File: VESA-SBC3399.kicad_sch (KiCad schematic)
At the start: 0 parts

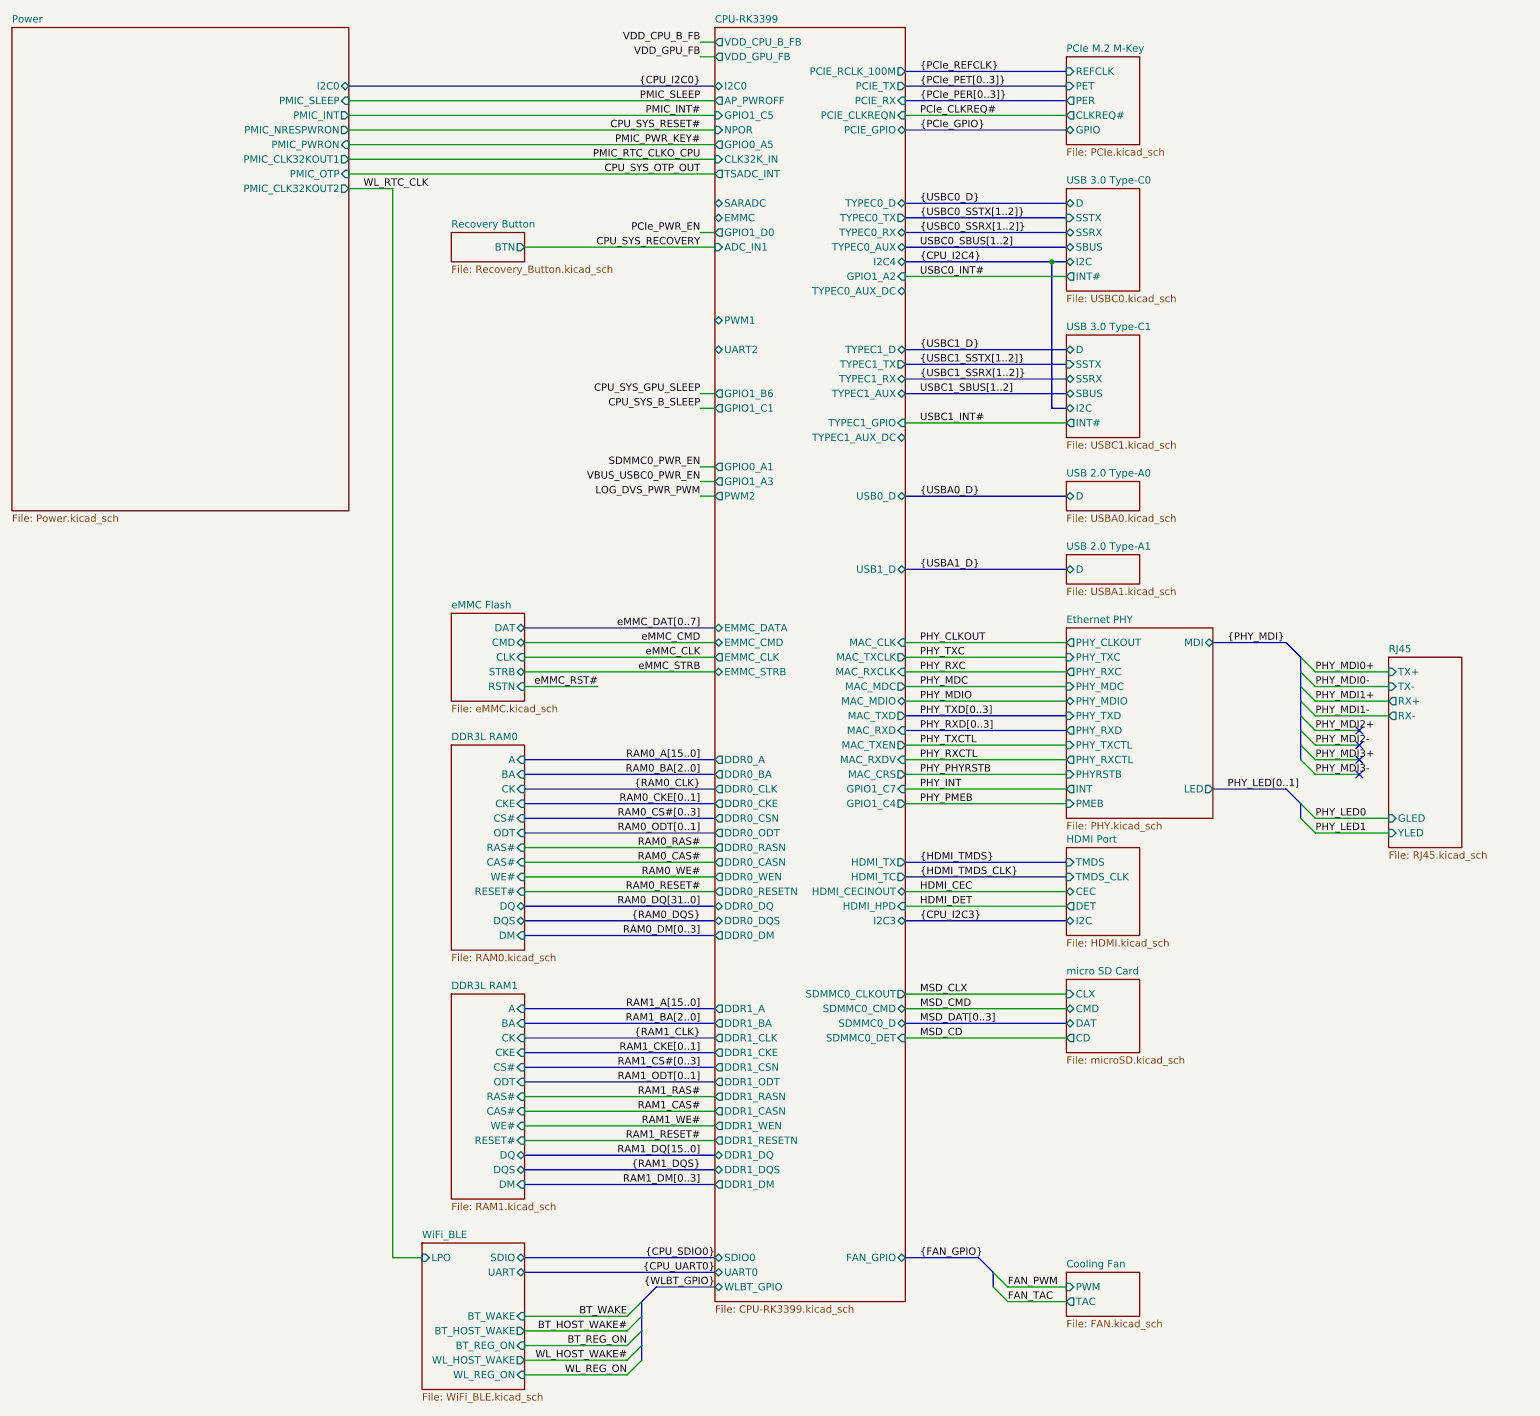
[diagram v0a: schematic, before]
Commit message: update design power
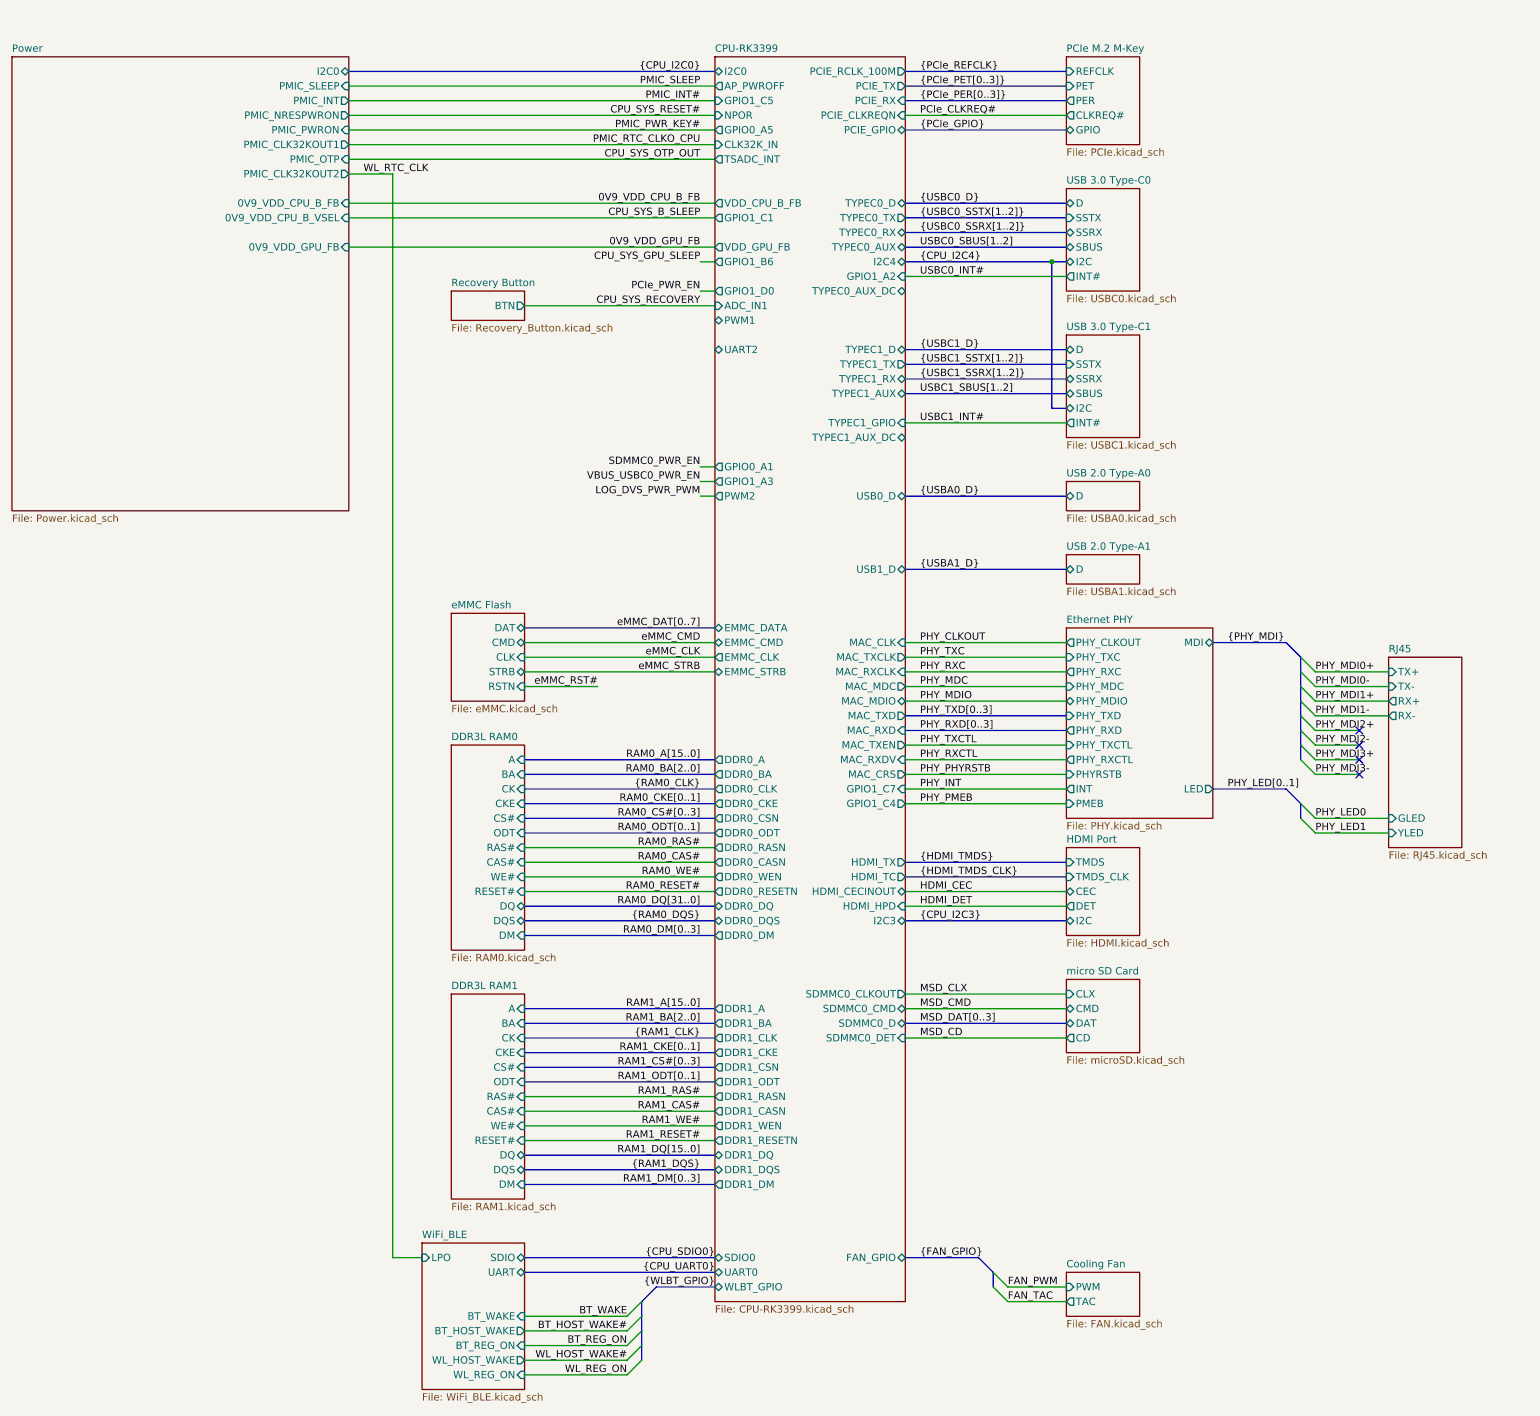
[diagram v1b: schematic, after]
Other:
- sheet CPU-RK3399 ports: added none; removed EMMC, SARADC
- sheet Power ports: added 0V9_VDD_CPU_B_FB, 0V9_VDD_CPU_B_VSEL, 0V9_VDD_GPU_FB; removed none
